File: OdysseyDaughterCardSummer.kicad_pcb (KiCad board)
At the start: 2 copper layers, 36.3 x 46.6 mm, 17 parts, among them J1 Conn_01x02, X1 OdysseyDaughterCard

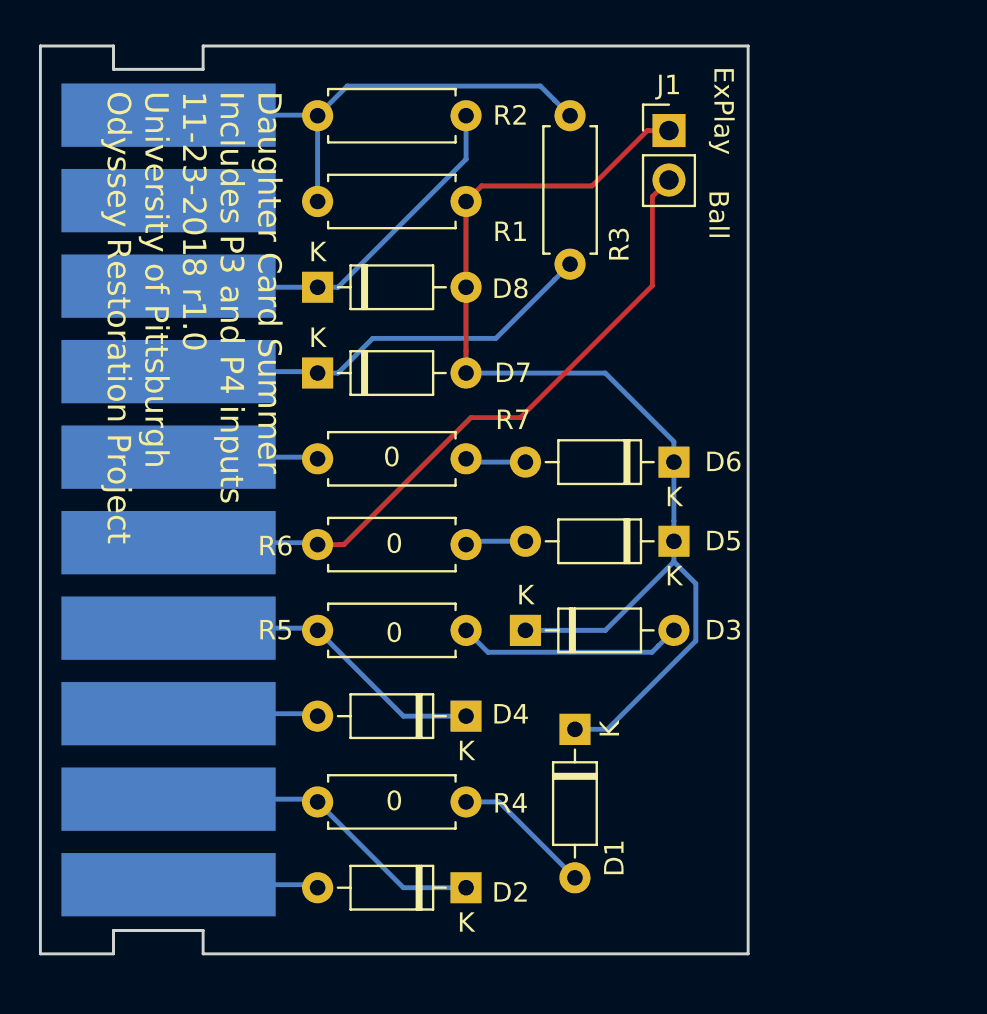
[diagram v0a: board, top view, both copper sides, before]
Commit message: R1.1 gerbs and board NTSC generator
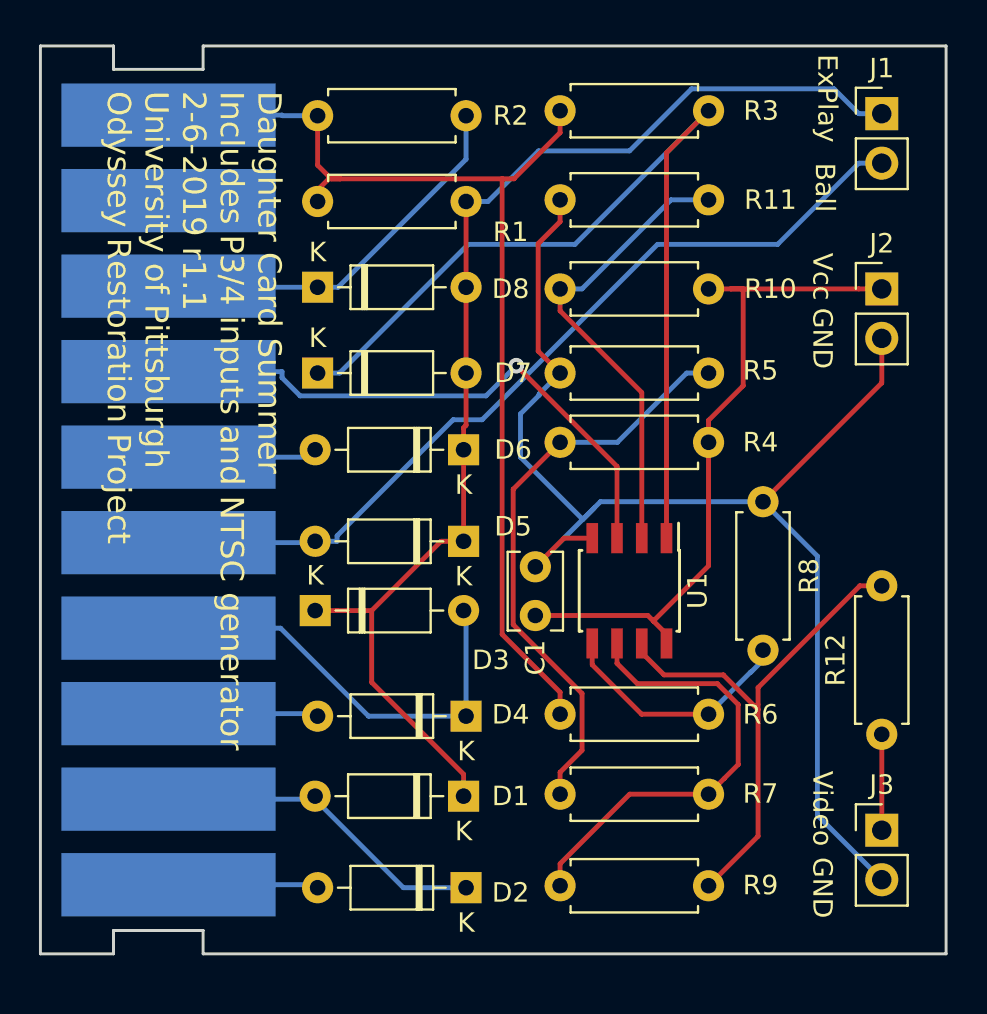
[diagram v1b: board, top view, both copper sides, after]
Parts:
- added C1: 0.1u, Capacitor_THT:C_Disc_D3.8mm_W2.6mm_P2.50mm, F.Cu at (147.8, 106.9)
- added J2: Conn_01x02, Connector_PinHeader_2.54mm:PinHeader_1x02_P2.54mm_Vertical, F.Cu at (165.6, 90.2)
- added J3: Conn_Coaxial, Connector_PinHeader_2.54mm:PinHeader_1x02_P2.54mm_Vertical, F.Cu at (165.6, 118.0)
- added R10: 4.7k, Resistor_THT:R_Axial_DIN0207_L6.3mm_D2.5mm_P7.62mm_Horizontal, F.Cu at (156.7, 90.2)
- added R11: 1k, Resistor_THT:R_Axial_DIN0207_L6.3mm_D2.5mm_P7.62mm_Horizontal, F.Cu at (156.7, 85.6)
- added R12: 75, Resistor_THT:R_Axial_DIN0207_L6.3mm_D2.5mm_P7.62mm_Horizontal, F.Cu at (165.6, 113.0)
- added R8: 100k, Resistor_THT:R_Axial_DIN0207_L6.3mm_D2.5mm_P7.62mm_Horizontal, F.Cu at (159.5, 101.1)
- added R9: 100k, Resistor_THT:R_Axial_DIN0207_L6.3mm_D2.5mm_P7.62mm_Horizontal, F.Cu at (156.7, 120.8)
- added U1: TLV3542, Package_SO:SOIC-8_3.9x4.9mm_P1.27mm, F.Cu at (152.7, 105.7)
- R4: value 0 -> 4.7k
- R5: value 0 -> 820
- R6, R7: value 0 -> 33k
- moved R7 26.4 mm to (156.7, 116.1), turned to 180 degrees
- moved R4 22.3 mm to (149.1, 98.0)
- moved R6 21.9 mm to (156.7, 112.0), turned to 180 degrees
- moved R5 18.1 mm to (149.1, 94.5)
- moved J1 11.0 mm to (165.6, 81.2)
- moved D3 10.8 mm to (136.5, 106.7)
- moved D6 10.8 mm to (144.1, 98.4)
- moved D5 10.8 mm to (144.1, 103.1)
- moved R3 10.6 mm to (156.7, 81.0), turned to 180 degrees
- moved D1 6.66 mm to (144.1, 116.2), turned to 180 degrees
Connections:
- D1 pad 2: Net-(D1-Pad2) -> /Card2
- D3 pad 2: Net-(D3-Pad2) -> /Card4
- D5 pad 2: Net-(D5-Pad2) -> /Card5
- D6 pad 2: Net-(D6-Pad2) -> /Card6
- D7 pad 1: /Card7 -> Net-(D7-Pad1)
- R3 pad 1: /Card7 -> Net-(D7-Pad1)
- R4 pad 1: /Card2 -> Net-(R4-Pad1)
- R4 pad 2: Net-(D1-Pad2) -> VCC
- R5 pad 1: /Card4 -> GND
- R5 pad 2: Net-(D3-Pad2) -> Net-(R4-Pad1)
- R6 pad 1: /Card5 -> Net-(R6-Pad1)
- R6 pad 2: Net-(D5-Pad2) -> /Card10
- R7 pad 1: /Card6 -> Net-(R7-Pad1)
- R7 pad 2: Net-(D6-Pad2) -> Net-(R4-Pad1)
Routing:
- net GND: track 0.00 -> 69.8 mm
- net Net-(D7-Pad1): track 0.00 -> 48.5 mm
- net VCC: track 0.00 -> 36.1 mm
- net Net-(R4-Pad1): track 0.00 -> 30.1 mm
- net /Card10: track 26.3 -> 55.8 mm
- net Net-(R12-Pad2): track 0.00 -> 27.4 mm
- net Net-(R10-Pad2): track 0.00 -> 24.0 mm
- net Net-(R7-Pad1): track 0.00 -> 23.6 mm
- net Net-(R6-Pad1): track 0.00 -> 12.6 mm
- net Net-(D3-Pad2): track 11.6 -> 0.00 mm
- net /Card5: track 36.2 -> 45.1 mm
- net /Card7: track 23.0 -> 30.2 mm, vias 0 -> 1
- net Net-(D1-Pad2): track 7.20 -> 0.00 mm
- net /Card4: track 17.1 -> 22.6 mm
- net Net-(J3-Pad1): track 0.00 -> 4.92 mm
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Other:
- board size 36.3 x 46.6 mm -> 46.5 x 46.6 mm
- board text added: "Daughter Card Summer Includes P3/4 inputs and NTSC generator 2-6-2019 r1.1 University of Pittsburgh Odyssey Restoration Project"
- board text added: "GND"
- board text added: "Vcc"
- board text added: "Video"
- board text removed: "Daughter Card Summer Includes P3 and P4 inputs 11-23-2018 r1.0 University of Pittsburgh Odyssey Restoration Project"
